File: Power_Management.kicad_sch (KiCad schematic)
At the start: 16 parts, among them J17 3V_Selection_Header, J26 USB_B_Micro, J4 JST_XH_2.54_Plug, J8 Power_Selector_Jumper, Q2 MOSFET_SI2333DDS-T1-BE3, U5 USBLC6-2SC6

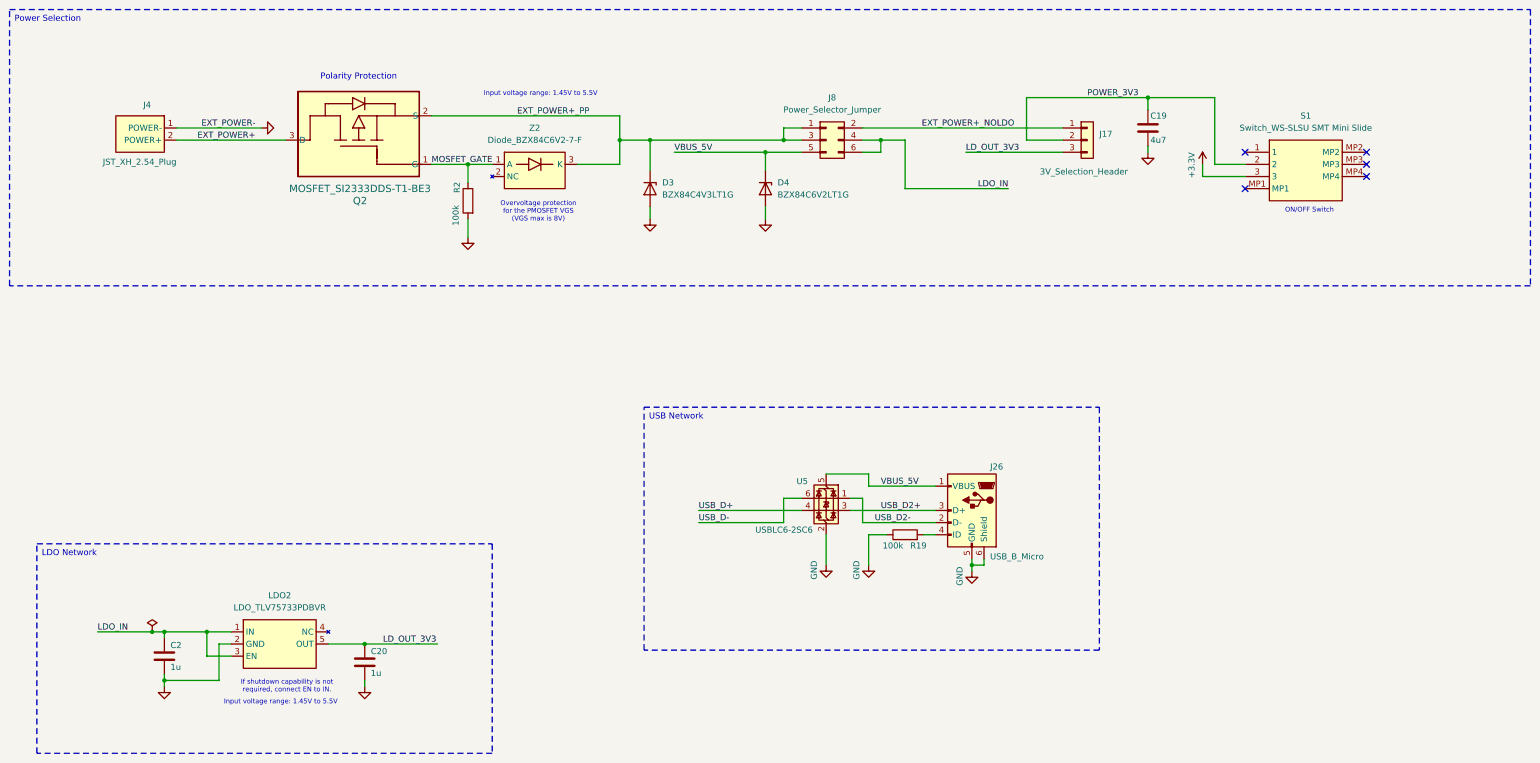
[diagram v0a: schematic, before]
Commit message: Update
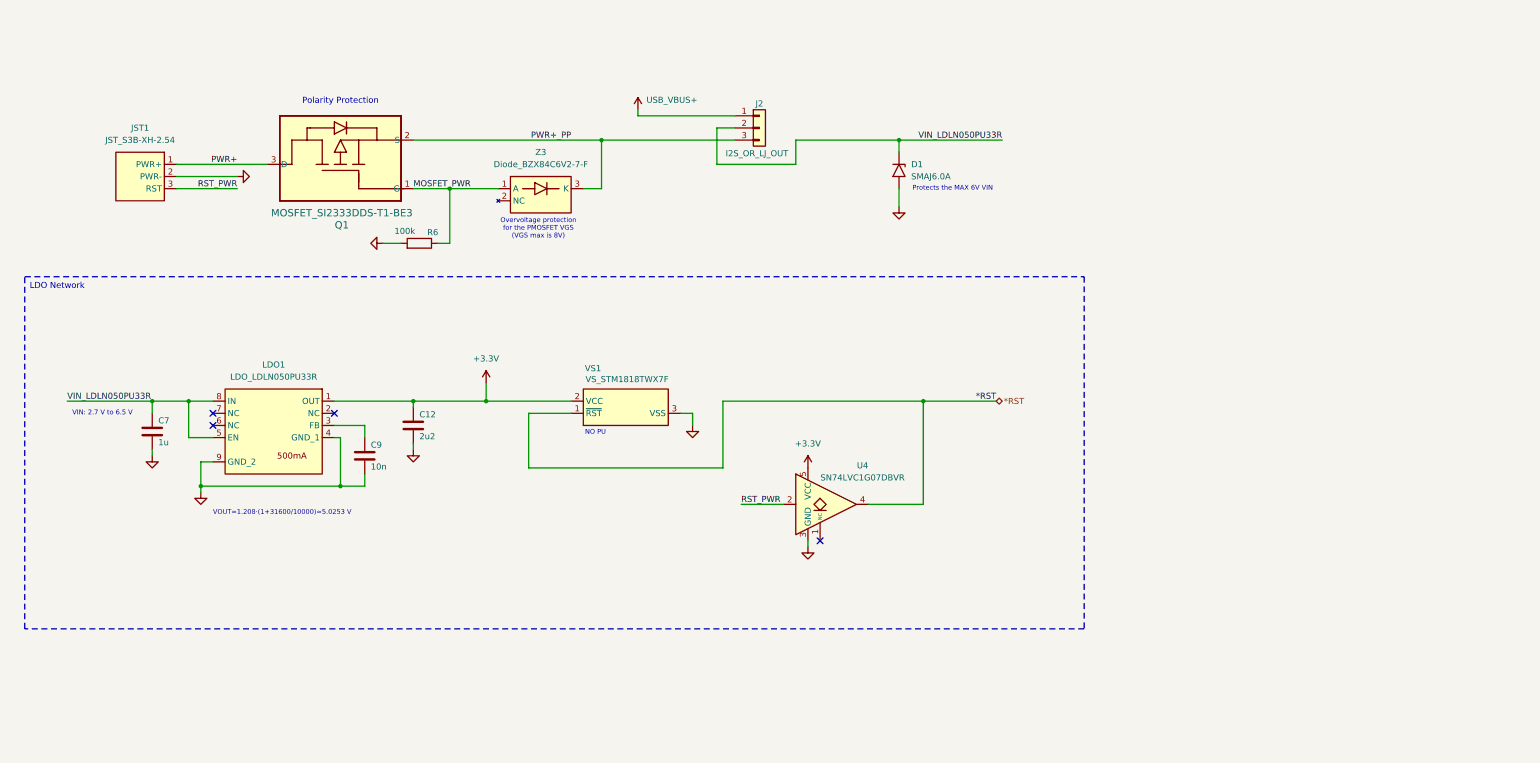
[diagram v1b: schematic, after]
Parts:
- removed C19: 4u7, Capacitor_SMD:C_0805_2012Metric, symbol Device:C
- removed C2, C20: 1u, Capacitor_SMD:C_0805_2012Metric, symbol Device:C
- removed D3: BZX84C4V3LT1G, Package_TO_SOT_SMD:SOT-23, symbol Diode:BZX84Cxx
- removed D4: BZX84C6V2LT1G, Package_TO_SOT_SMD:SOT-23, symbol Diode:BZX84Cxx
- removed J17: 3V_Selection_Header, Connector_PinHeader_2.54mm:PinHeader_1x03_P2.54mm_Vertical, symbol Connector_Generic:Conn_01x03
- removed J26: USB_B_Micro, Connector_USB:USB_Micro-B_XKB_U254-051T-4BH83-F1S, symbol Connector:USB_B_Micro
- removed J4: JST_XH_2.54_Plug, Personal_Project:Connector_Power2pin_SHDRRA2W80P0X250_1X2_740X1150X610P, symbol Personal_Projects:Connector_Power2pin_JST_XH_2.54_Plug
- removed J8: Power_Selector_Jumper, Connector_PinHeader_2.54mm:PinHeader_2x03_P2.54mm_Vertical, symbol Connector_Generic:Conn_02x03_Odd_Even
- removed LDO2: LDO_TLV75733PDBVR, Personal_Project:LDO_SOT95P280X145-5N, symbol Personal_Projects:LDO_TLV75733PDBVR
- removed Q2: MOSFET_SI2333DDS-T1-BE3, Personal_Project:MOSFET_ SI2333DDS_SOT_DS-T1-BE3_VIS, symbol Personal_Projects:MOSFET_SI2333DDS-T1-BE3
- removed R19, R2: 100k, Resistor_SMD:R_0805_2012Metric, symbol Device:R
- removed S1: Switch_WS-SLSU SMT Mini Slide, Personal_Project:Switch_WS-SLSU SMT Mini Slide, symbol Personal_Projects:Switch_WS-SLSU SMT Mini Slide
- removed U5: USBLC6-2SC6, Package_TO_SOT_SMD:SOT-23-6, symbol Power_Protection:USBLC6-2SC6
- removed Z2: Diode_BZX84C6V2-7-F, Personal_Project:Diode_BZX84C6V2_SOT96P240X110-3N, symbol Personal_Projects:Diode_BZX84C6V2-7-F
- added C12: 2u2, Capacitor_SMD:C_0805_2012Metric, symbol Device:C
- added C7: 1u, Capacitor_SMD:C_0805_2012Metric, symbol Device:C
- added C9: 10n, Capacitor_SMD:C_0805_2012Metric, symbol Device:C
- added D1: SMAJ6.0A, Personal_Project:DO-214AC-2, symbol Personal_Projects:DIODE_SMAJ6.0A
- added J2: I2S_OR_LJ_OUT, Connector_PinHeader_2.54mm:PinHeader_1x03_P2.54mm_Vertical, symbol Connector_Generic:Conn_01x03
- added JST1: JST_S3B-XH-2.54, Personal_Project:JST_S3B-XH-SHDRRA3W64P0X250_1X3_990X1150X610P, symbol Personal_Projects:JST_S3B-XH-A-1_LF_SN
- added LDO1: LDO_LDLN050PU33R, Package_DFN_QFN:DFN-8-1EP_3x3mm_P0.65mm_EP1.7x2.05mm, symbol Personal_Projects:LDO_LDLN050PUR
- added Q1: MOSFET_SI2333DDS-T1-BE3, Personal_Project:MOSFET_ SI2333DDS_SOT_DS-T1-BE3_VIS, symbol Personal_Projects:MOSFET_SI2333DDS-T1-BE3
- added R6: 100k, Resistor_SMD:R_0805_2012Metric, symbol Device:R
- added U4: SN74LVC1G07DBVR, Package_TO_SOT_SMD:SOT-23-5, symbol 74xGxx:74LVC1G07
- added VS1: VS_STM1818TWX7F, Personal_Project:SOT-23-3_SOT103P237X112-3N, symbol Personal_Projects:VS_STM1813LWX7F
- added Z3: Diode_BZX84C6V2-7-F, Personal_Project:Diode_BZX84C6V2_SOT96P240X110-3N, symbol Personal_Projects:Diode_BZX84C6V2-7-F
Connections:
- net +3.3V: now also C12.1, LDO1.1 (OUT), U4.5 (VCC), VS1.2 (VCC)
- net GND: now also C12.2, C7.2, C9.2, D1.2 (A), JST1.2 (PWR-), LDO1.4 (GND_1), LDO1.9 (GND_2), R6.2, U4.3 (GND), VS1.3 (VSS)
- new net: C9.1, LDO1.3 (FB)
- new net *RST: U4.4, VS1.1 (~{RST})
- new net MOSFET_PWR: Q1.1 (G), R6.1, Z3.1 (A)
- new net PWR+: JST1.1 (PWR+), Q1.3 (D)
- new net PWR+_PP: J2.3 (Pin_3), Q1.2 (S), Z3.3 (K)
- new net RST_PWR: JST1.3 (RST), U4.2
- new net USB_VBUS+: J2.1 (Pin_1)
- new net VIN_LDLN050PU33R: C7.1, D1.1 (K), J2.2 (Pin_2), LDO1.5 (EN), LDO1.8 (IN)
- no-connect marks 5 -> 4
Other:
- note added: "NO PU"
- note added: "Protects the MAX 6V VIN"
- note added: "VIN: 2.7 V to 6.5 V"
- note added: "VOUT​=1.208⋅(1+31600/10000)≈5.0253 V"
- note removed: "If shutdown capability is not required, connect EN to IN."
- note removed: "Input voltage range: 1.45V to 5.5V"
- note removed: "ON/OFF Switch"

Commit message: Update
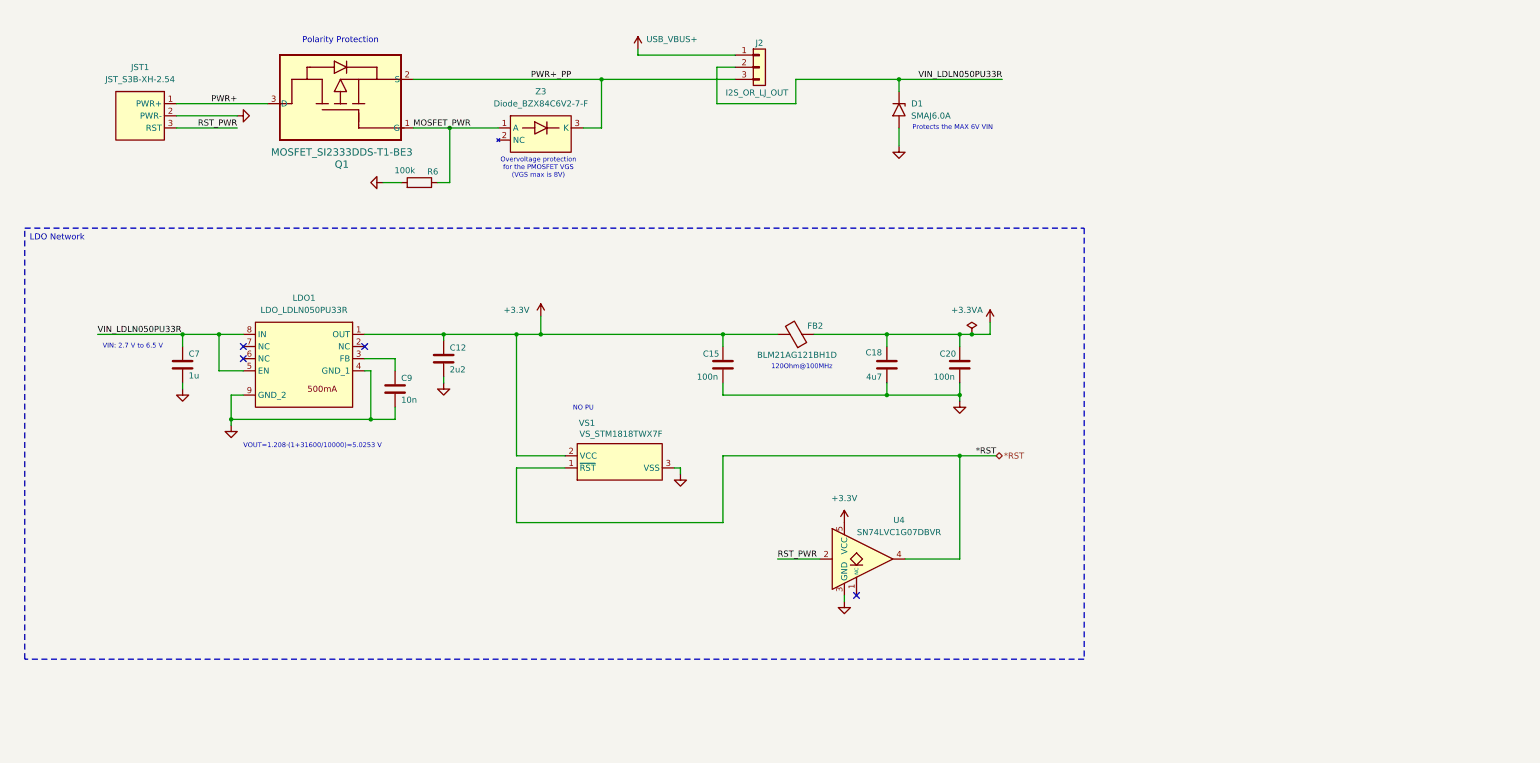
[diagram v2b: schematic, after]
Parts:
- added C15, C20: 100n, Capacitor_SMD:C_0805_2012Metric, symbol Device:C
- added C18: 4u7, Capacitor_SMD:C_0805_2012Metric, symbol Device:C
- added FB2: BLM21AG121BH1D, Capacitor_SMD:C_0805_2012Metric, symbol Device:FerriteBead
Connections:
- net +3.3V: now also C15.1, FB2.2
- net GND: now also C15.2, C18.2, C20.2
- new net +3.3VA: C18.1, C20.1, FB2.1
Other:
- note added: "120Ohm@100MHz"
- moved on the sheet: C12, C7, C9, D1, J2, JST1, LDO1, Q1, R6, U4, VS1, Z3
